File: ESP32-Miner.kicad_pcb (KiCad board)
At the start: 2 copper layers, 32 x 32 mm, 28 parts, among them J1 EXP, J2 PROGRAM, Q1 BSS138, Q2 BSS138, SW1 RESET, SW2 BOOT, U1 AMS1117-3.3, U2 ESP32-WROOM-32D

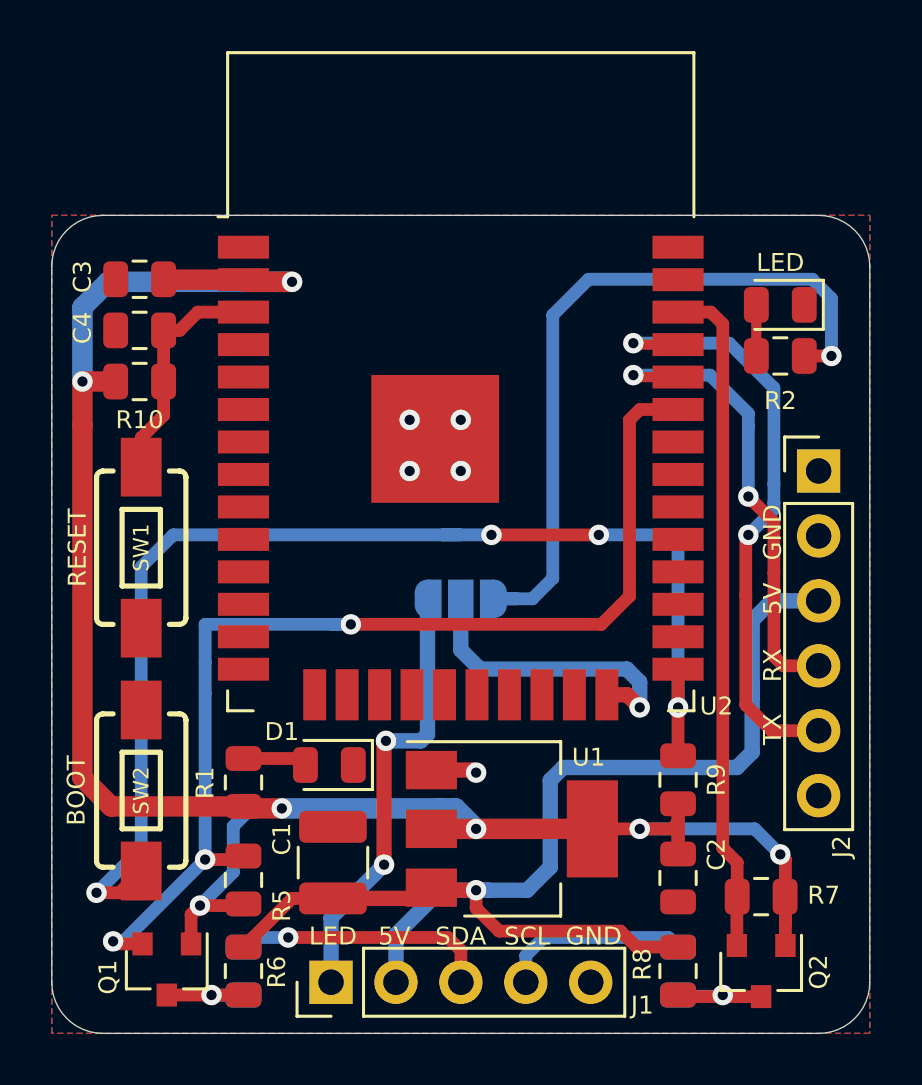
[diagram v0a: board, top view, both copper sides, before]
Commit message: Updated project for KiCad 7 & added Gerber files
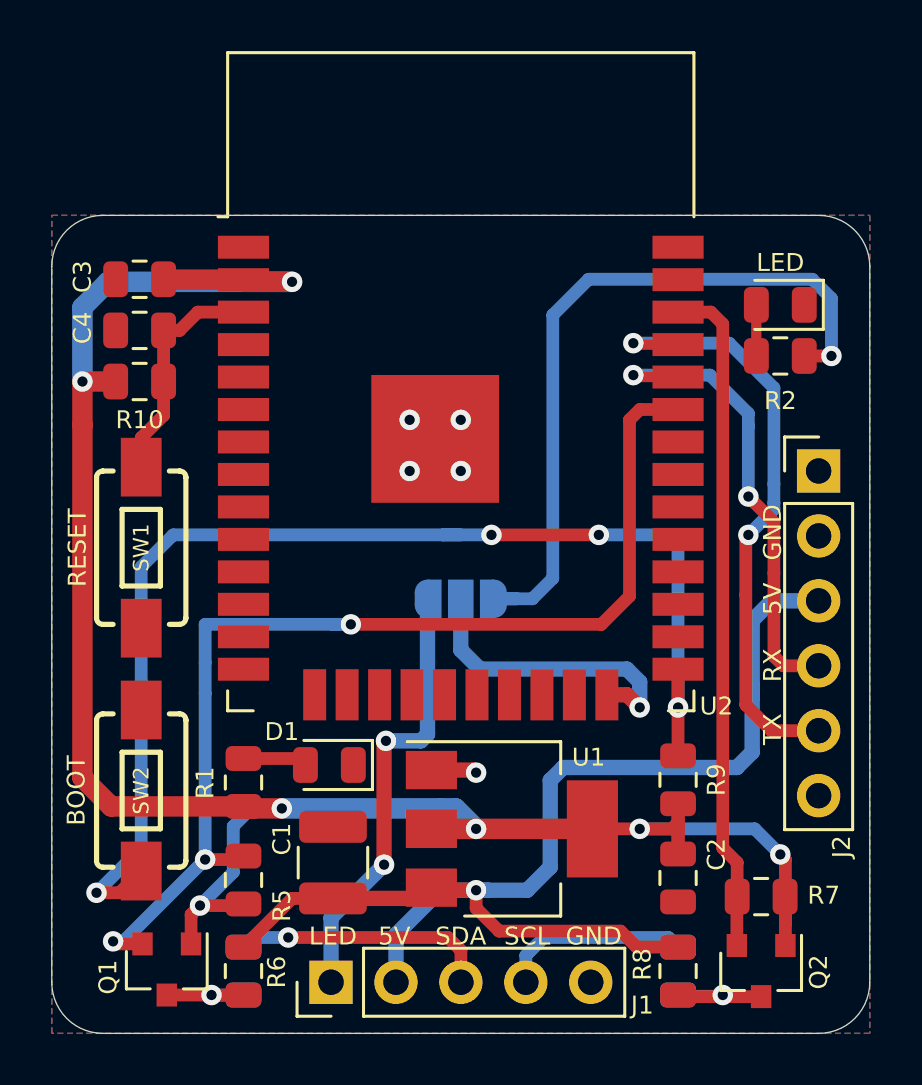
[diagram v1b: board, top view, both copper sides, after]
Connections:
- J2 pad 1: Net-(J2-Pad1) -> unconnected-(J2-Pin_1-Pad1)
- J2 pad 6: Net-(J2-Pad6) -> unconnected-(J2-Pin_6-Pad6)
- U2 pad 10: Net-(U2-Pad10) -> unconnected-(U2-IO25-Pad10)
- U2 pad 11: Net-(U2-Pad11) -> unconnected-(U2-IO26-Pad11)
- U2 pad 12: Net-(U2-Pad12) -> unconnected-(U2-IO27-Pad12)
- U2 pad 13: Net-(U2-Pad13) -> unconnected-(U2-IO14-Pad13)
- U2 pad 14: Net-(U2-Pad14) -> unconnected-(U2-IO12-Pad14)
- U2 pad 16: Net-(U2-Pad16) -> unconnected-(U2-IO13-Pad16)
- U2 pad 17: Net-(U2-Pad17) -> unconnected-(U2-SHD/SD2-Pad17)
- U2 pad 18: Net-(U2-Pad18) -> unconnected-(U2-SWP/SD3-Pad18)
- U2 pad 19: Net-(U2-Pad19) -> unconnected-(U2-SCS/CMD-Pad19)
- U2 pad 20: Net-(U2-Pad20) -> unconnected-(U2-SCK/CLK-Pad20)
- U2 pad 21: Net-(U2-Pad21) -> unconnected-(U2-SDO/SD0-Pad21)
- U2 pad 22: Net-(U2-Pad22) -> unconnected-(U2-SDI/SD1-Pad22)
- U2 pad 23: Net-(U2-Pad23) -> unconnected-(U2-IO15-Pad23)
- U2 pad 26: Net-(U2-Pad26) -> unconnected-(U2-IO4-Pad26)
- U2 pad 27: Net-(U2-Pad27) -> unconnected-(U2-IO16-Pad27)
- U2 pad 28: Net-(U2-Pad28) -> unconnected-(U2-IO17-Pad28)
- U2 pad 29: Net-(U2-Pad29) -> unconnected-(U2-IO5-Pad29)
- U2 pad 30: Net-(U2-Pad30) -> unconnected-(U2-IO18-Pad30)
- U2 pad 31: Net-(U2-Pad31) -> unconnected-(U2-IO19-Pad31)
- U2 pad 32: Net-(U2-Pad32) -> unconnected-(U2-NC-Pad32)
- U2 pad 37: Net-(U2-Pad37) -> unconnected-(U2-IO23-Pad37)
- U2 pad 4: Net-(U2-Pad4) -> unconnected-(U2-SENSOR_VP-Pad4)
- U2 pad 5: Net-(U2-Pad5) -> unconnected-(U2-SENSOR_VN-Pad5)
- U2 pad 6: Net-(U2-Pad6) -> unconnected-(U2-IO34-Pad6)
- U2 pad 7: Net-(U2-Pad7) -> unconnected-(U2-IO35-Pad7)
- U2 pad 8: Net-(U2-Pad8) -> unconnected-(U2-IO32-Pad8)
- U2 pad 9: Net-(U2-Pad9) -> unconnected-(U2-IO33-Pad9)
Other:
- net class Default removed
